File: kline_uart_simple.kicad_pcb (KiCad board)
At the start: 4 copper layers, 36.8 x 19.3 mm, 9 parts, among them J1 USB2UART, J2 KLINE_CONN, Q1 BC547, Q2 BC547

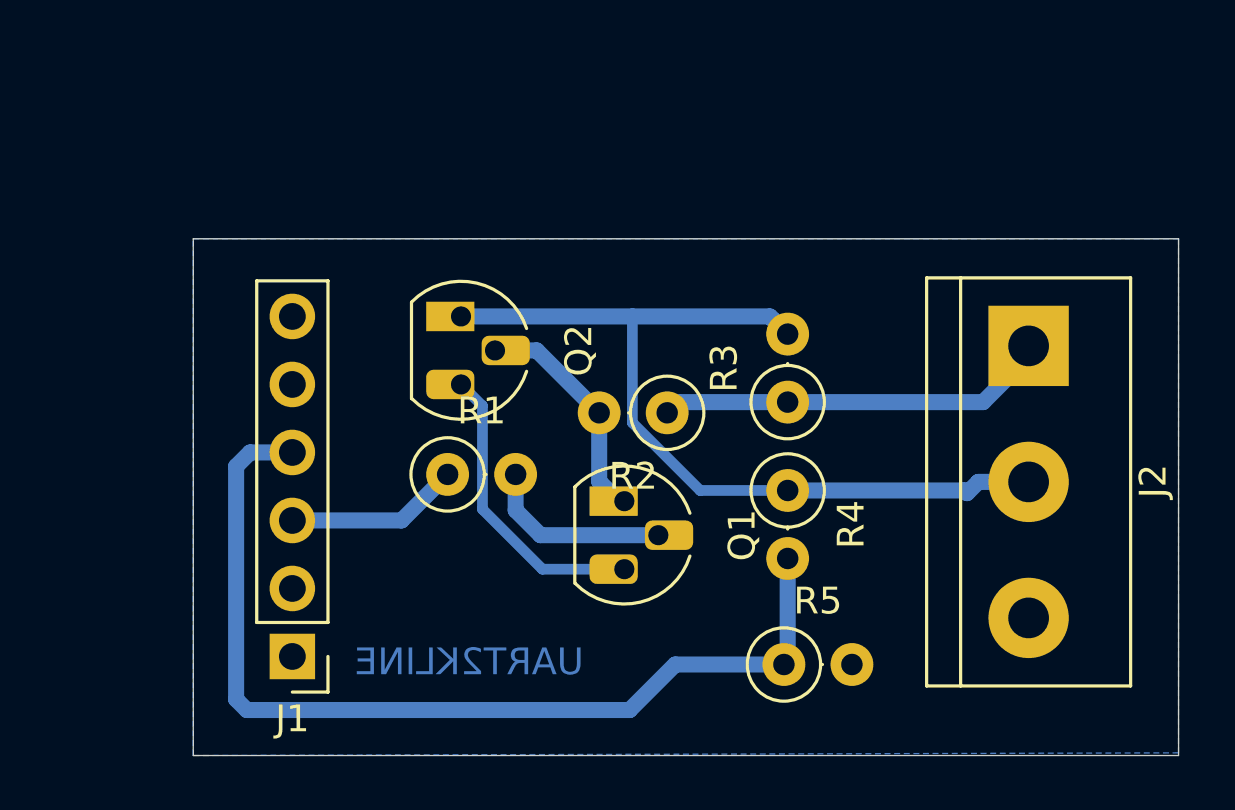
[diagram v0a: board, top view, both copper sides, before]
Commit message: New output files
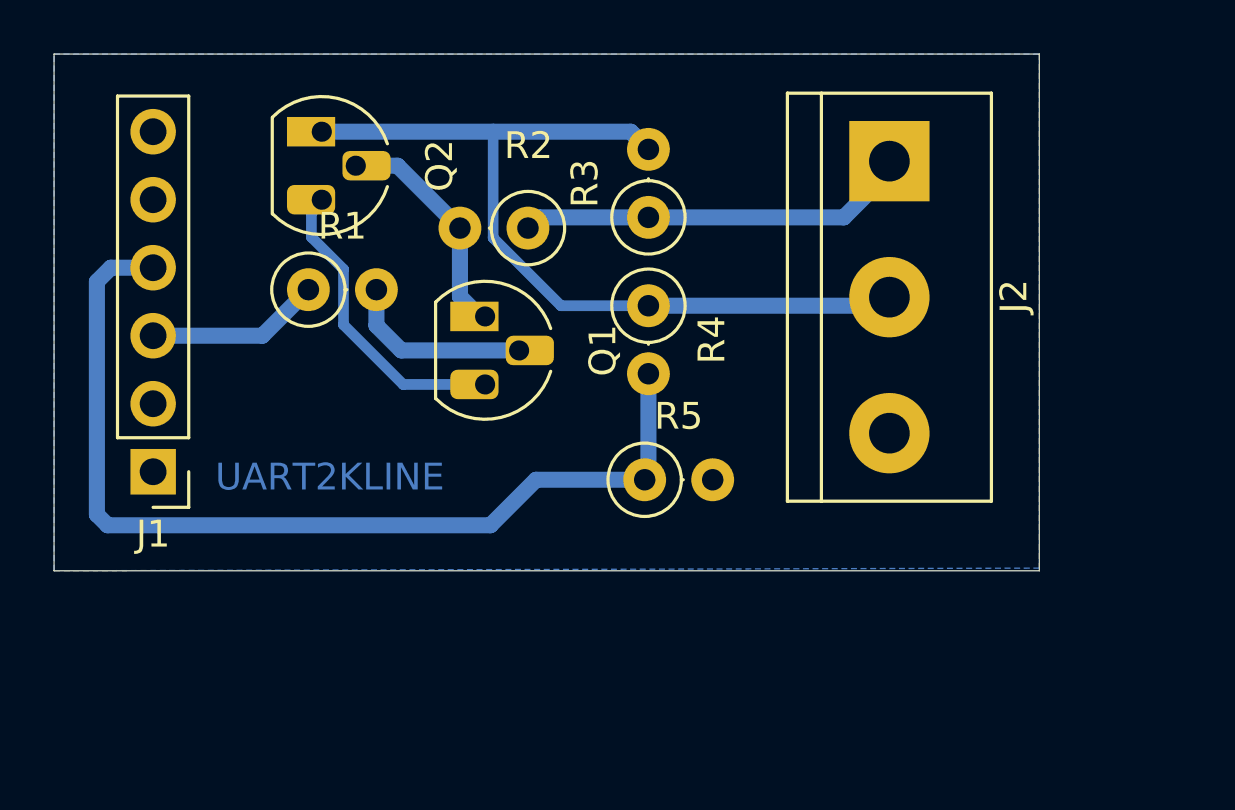
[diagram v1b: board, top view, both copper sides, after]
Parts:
- moved R4 8.64 mm to (32.3, 19.4)
- moved J2 8.64 mm to (41.3, 14.0)
- moved R3 8.64 mm to (32.3, 16.1)
- moved R5 8.64 mm to (32.2, 25.9)
- moved Q2 8.64 mm to (20.1, 12.9)
- moved J1 8.64 mm to (13.8, 25.6)
- moved Q1 8.64 mm to (26.2, 19.8)
- moved R1 8.64 mm to (19.6, 18.8)
- moved R2 8.64 mm to (27.8, 16.5)
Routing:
- net KLINE: track 34.3 -> 33.8 mm
